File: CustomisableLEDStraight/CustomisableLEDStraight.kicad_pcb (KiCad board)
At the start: 2 copper layers, 98 x 8 mm, 16 parts, among them J1 Conn_01x05_Socket, J2 Conn_01x05_Socket, J3 Conn_01x05_Socket, J4 Conn_01x05_Socket, J5 Conn_01x05_Socket, J6 Conn_01x05_Socket

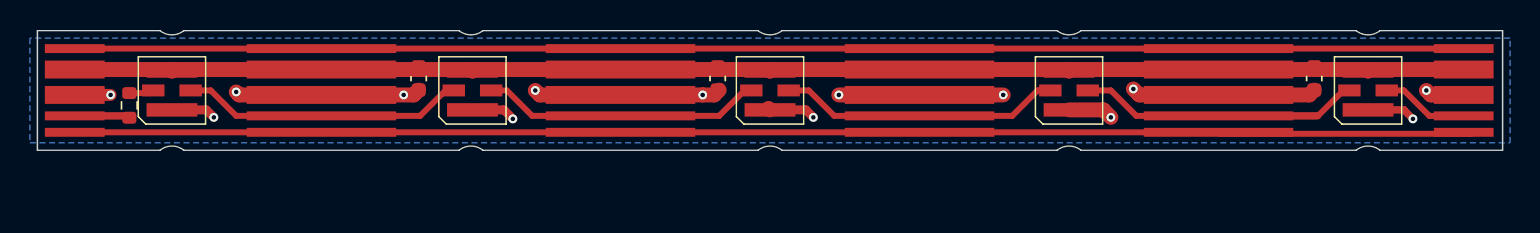
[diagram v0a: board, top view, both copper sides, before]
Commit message: added readme to project
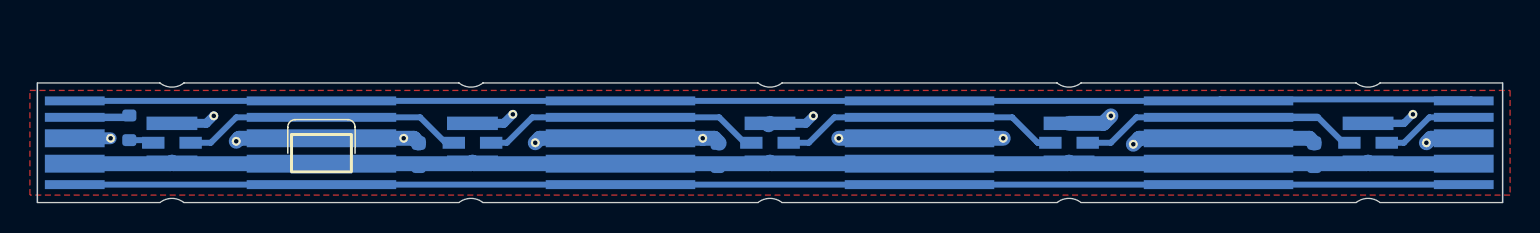
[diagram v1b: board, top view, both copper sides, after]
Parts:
- C1, C2, C3, D1, D2, D3, D4, D5, J1, J2, J3, J4, J5, J6, R1: moved to B.Cu
- ESKI1: moved to F.Cu
- moved C1 5.10 mm to (66.5, 79.3), turned to -90 degrees
- moved C2 5.10 mm to (86.5, 79.3), turned to -90 degrees
- moved C3 5.10 mm to (126.4, 79.3), turned to -90 degrees
- moved ESKI1 3.85 mm to (60.0, 80.5), turned to 0 degrees
- moved D1 3.50 mm to (50.0, 78.5)
- moved D2 3.50 mm to (70.1, 78.5)
- moved D3 3.50 mm to (90.0, 78.5)
- moved D4 3.50 mm to (110.0, 78.5)
- moved D5 3.50 mm to (130.0, 78.5)
- moved J1 3.50 mm to (43.5, 78.5)
- moved J2 3.50 mm to (60.0, 78.5)
- moved J3 3.50 mm to (80.0, 78.5)
- moved J4 3.50 mm to (100.0, 78.5)
- moved J5 3.50 mm to (120.0, 78.5)
- moved J6 3.50 mm to (136.4, 78.5)
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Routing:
- added copper zone on F.Cu, net GND
- removed copper zone on B.Cu, net GND
